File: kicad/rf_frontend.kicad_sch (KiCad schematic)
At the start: 5 parts, among them U10 LTC2311-16

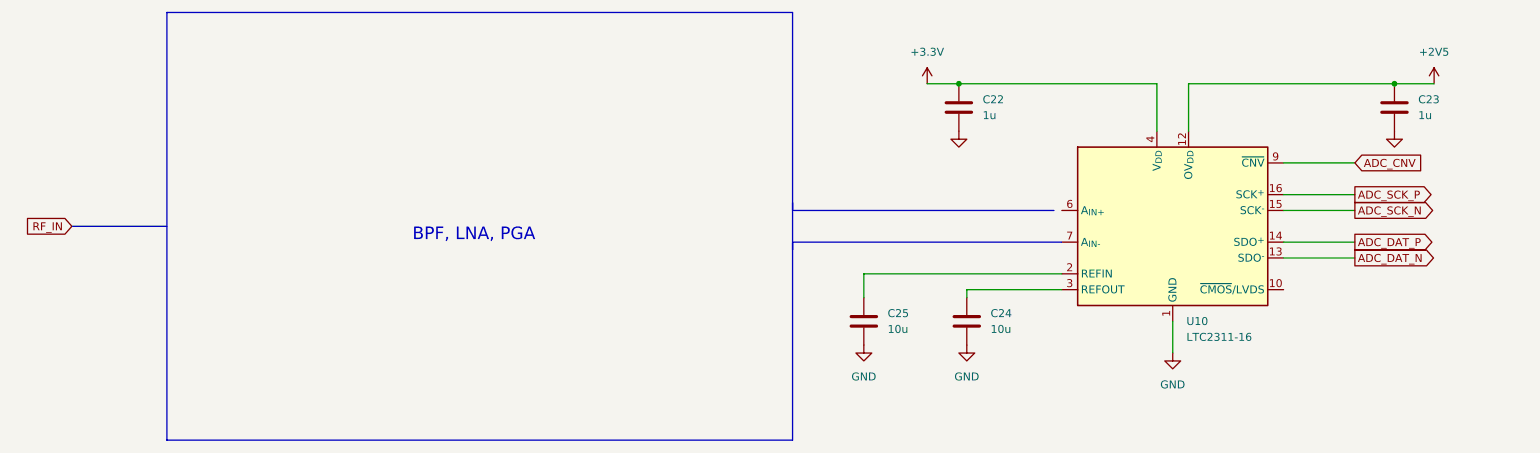
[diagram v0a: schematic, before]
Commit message: updates
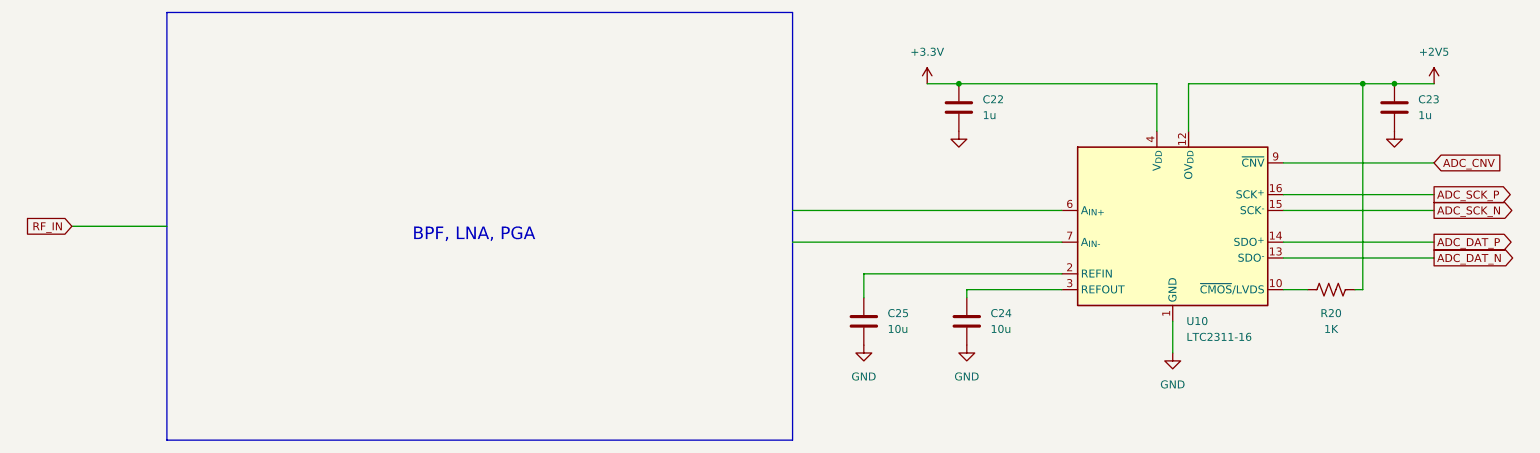
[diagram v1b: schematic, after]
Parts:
- added R20: 1K, symbol Device:R_US
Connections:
- net +2V5: now also R20.2
- net at U10.10 (~{CMOS}/LVDS): now also R20.1
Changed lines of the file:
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@@
   (junction (at 241.3 111.76) (diameter 0) (color 0 0 0 0)
   )
+  (junction (at 306.07 111.76) (diameter 0) (color 0 0 0 0)
+  )
+  (wire (pts (xy 304.8 144.78) (xy 306.07 144.78))
+    (stroke (width 0) (type default))
+  )
+  (wire (pts (xy 293.37 144.78) (xy 297.18 144.78))
+    (stroke (width 0) (type default))
+  )
   (wire (pts (xy 257.81 144.78) (xy 242.57 144.78))
     (stroke (width 0) (type default))
   )
+  (wire (pts (xy 306.07 111.76) (xy 311.15 111.76))
+    (stroke (width 0) (type default))
+  )
   (wire (pts (xy 226.06 142.24) (xy 226.06 146.05))
     (stroke (width 0) (type default))
@@
     (stroke (width 0) (type default))
   )
-  (wire (pts (xy 293.37 129.54) (xy 304.8 129.54))
-    (stroke (width 0) (type default))
-  )
-  (bus (pts (xy 214.63 137.16) (xy 214.63 138.43))
+  (wire (pts (xy 99.06 134.62) (xy 114.3 134.62))
+    (stroke (width 0) (type default))
+  )
+  (wire (pts (xy 293.37 129.54) (xy 317.5 129.54))
+    (stroke (width 0) (type default))
+  )
+  (wire (pts (xy 214.63 132.08) (xy 257.81 132.08))
     (stroke (width 0) (type default))
   )
@@
     (stroke (width 0) (type default))
   )
-  (bus (pts (xy 257.81 137.16) (xy 214.63 137.16))
-    (stroke (width 0) (type default))
-  )
-  (bus (pts (xy 99.06 134.62) (xy 114.3 134.62))
-    (stroke (width 0) (type default))
-  )
-  (wire (pts (xy 278.13 111.76) (xy 311.15 111.76))
+  (wire (pts (xy 278.13 111.76) (xy 306.07 111.76))
     (stroke (width 0) (type default))
   )
@@
     (stroke (width 0) (type default))
   )
-  (wire (pts (xy 293.37 139.7) (xy 304.8 139.7))
+  (wire (pts (xy 306.07 111.76) (xy 306.07 144.78))
+    (stroke (width 0) (type default))
+  )
+  (wire (pts (xy 293.37 139.7) (xy 317.5 139.7))
     (stroke (width 0) (type default))
   )
@@
     (stroke (width 0) (type default))
   )
-  (wire (pts (xy 293.37 137.16) (xy 304.8 137.16))
+  (wire (pts (xy 293.37 137.16) (xy 317.5 137.16))
+    (stroke (width 0) (type default))
+  )
+  (wire (pts (xy 214.63 137.16) (xy 257.81 137.16))
     (stroke (width 0) (type default))
   )
@@
     (stroke (width 0) (type default))
   )
-  (wire (pts (xy 293.37 124.46) (xy 304.8 124.46))
-    (stroke (width 0) (type default))
-  )
-  (bus (pts (xy 256.54 132.08) (xy 214.63 132.08))
+  (wire (pts (xy 293.37 124.46) (xy 317.5 124.46))
     (stroke (width 0) (type default))
   )
@@
     (stroke (width 0) (type default))
   )
-  (bus (pts (xy 214.63 130.81) (xy 214.63 132.08))
-    (stroke (width 0) (type default))
-  )
-  (wire (pts (xy 293.37 132.08) (xy 304.8 132.08))
+  (wire (pts (xy 293.37 132.08) (xy 317.5 132.08))
     (stroke (width 0) (type default))
   )
@@
     (effects (font (size 2 2)) (justify left bottom))
   )
-  (global_label "ADC_DAT_N" (shape output) (at 304.8 139.7 0) (fields_autoplaced)
-    (effects (font (size 1.27 1.27)) (justify left))
-    (property "Intersheetrefs" "${INTERSHEET_REFS}" (at 318.0057 139.7 0)
-      (effects (font (size 1.27 1.27)) (justify left) hide)
-    )
-  )
-  (global_label "ADC_SCK_P" (shape output) (at 304.8 129.54 0) (fields_autoplaced)
-    (effects (font (size 1.27 1.27)) (justify left))
-    (property "Intersheetrefs" "${INTERSHEET_REFS}" (at 318.3685 129.54 0)
-      (effects (font (size 1.27 1.27)) (justify left) hide)
-    )
-  )
-  (global_label "ADC_DAT_P" (shape output) (at 304.8 137.16 0) (fields_autoplaced)
-    (effects (font (size 1.27 1.27)) (justify left))
-    (property "Intersheetrefs" "${INTERSHEET_REFS}" (at 317.9452 137.16 0)
+  (global_label "ADC_DAT_N" (shape output) (at 317.5 139.7 0) (fields_autoplaced)
+    (effects (font (size 1.27 1.27)) (justify left))
+    (property "Intersheetrefs" "${INTERSHEET_REFS}" (at 330.7057 139.7 0)
+      (effects (font (size 1.27 1.27)) (justify left) hide)
+    )
+  )
+  (global_label "ADC_SCK_P" (shape output) (at 317.5 129.54 0) (fields_autoplaced)
+    (effects (font (size 1.27 1.27)) (justify left))
+    (property "Intersheetrefs" "${INTERSHEET_REFS}" (at 331.0685 129.54 0)
+      (effects (font (size 1.27 1.27)) (justify left) hide)
+    )
+  )
+  (global_label "ADC_DAT_P" (shape output) (at 317.5 137.16 0) (fields_autoplaced)
+    (effects (font (size 1.27 1.27)) (justify left))
+    (property "Intersheetrefs" "${INTERSHEET_REFS}" (at 330.6452 137.16 0)
       (effects (font (size 1.27 1.27)) (justify left) hide)
     )
@@
     )
   )
-  (global_label "ADC_CNV" (shape input) (at 304.8 124.46 0) (fields_autoplaced)
-    (effects (font (size 1.27 1.27)) (justify left))
-    (property "Intersheetrefs" "${INTERSHEET_REFS}" (at 316.0705 124.46 0)
-      (effects (font (size 1.27 1.27)) (justify left) hide)
-    )
-  )
-  (global_label "ADC_SCK_N" (shape output) (at 304.8 132.08 0) (fields_autoplaced)
-    (effects (font (size 1.27 1.27)) (justify left))
-    (property "Intersheetrefs" "${INTERSHEET_REFS}" (at 318.429 132.08 0)
+  (global_label "ADC_CNV" (shape input) (at 317.5 124.46 0) (fields_autoplaced)
+    (effects (font (size 1.27 1.27)) (justify left))
+    (property "Intersheetrefs" "${INTERSHEET_REFS}" (at 328.7705 124.46 0)
+      (effects (font (size 1.27 1.27)) (justify left) hide)
+    )
+  )
+  (global_label "ADC_SCK_N" (shape output) (at 317.5 132.08 0) (fields_autoplaced)
+    (effects (font (size 1.27 1.27)) (justify left))
+    (property "Intersheetrefs" "${INTERSHEET_REFS}" (at 331.129 132.08 0)
       (effects (font (size 1.27 1.27)) (justify left) hide)
     )
@@
         )
       )
+    )
+  )
+  (symbol (lib_id "Device:R_US") (at 300.99 144.78 90) (unit 1)
+    (in_bom yes) (on_board yes) (dnp no)
+    (property "Reference" "R20" (at 300.99 148.59 90)
+      (effects (font (size 1.27 1.27)))
+    )
+    (property "Value" "1K" (at 300.99 151.13 90)
+      (effects (font (size 1.27 1.27)))
+    )
+    (property "Footprint" "" (at 301.244 143.764 90)
+      (effects (font (size 1.27 1.27)) hide)
+    )
+    (property "Datasheet" "~" (at 300.99 144.78 0)
+      (effects (font (size 1.27 1.27)) hide)
+    )
+    (pin "1")
+    (pin "2")
+    (instances
+      (project "gpsrx"
+        (path "/c3c549bc-9d82-4b6a-bdb9-a3870905229d/927dd695-6d3e-4555-8e99-f99aa71ecefd"
+          (reference "R20") (unit 1)
+        )
+      )
